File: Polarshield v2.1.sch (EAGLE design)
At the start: 82 parts, among them CN1 1X4-CLEANBIG, CN2 1X4-CLEANBIG, CN3 1X4-CLEANBIG, CN4 1X4-CLEANBIG, CN5 1X4-CLEANBIG, CN6 1X4-CLEANBIG, IC1 MP2307, IC2 74541PW, IC3 74541PW, IC4 74541PW, IC5 74541PW, J1 1X2-3.5MM, U1 ARDUINO_MEGA_SHIELD, X1 2.1MMJACKTHM

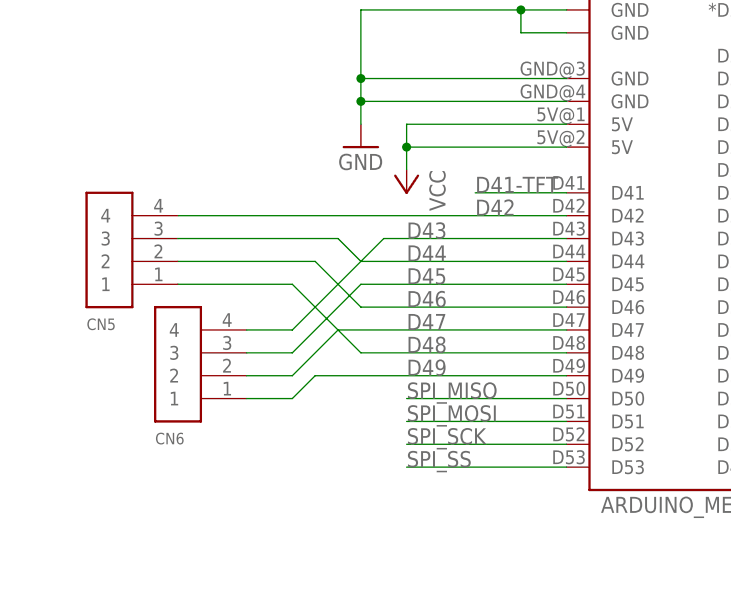
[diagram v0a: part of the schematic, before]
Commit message: Ran the DRU, ready for making.
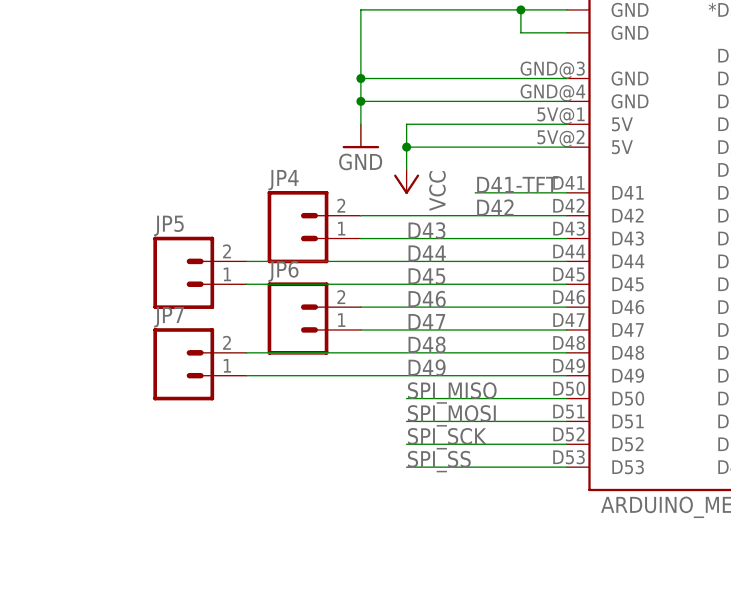
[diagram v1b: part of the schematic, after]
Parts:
- removed CN5, CN6: 1X4-CLEANBIG, Polarshield v2.0e:1X4-CLEANBIG
- added JP4, JP5, JP6, JP7: (no value), SparkFun-Connectors:M02POGO_PIN_HOLES_ONLY
- JP1, JP3: device SparkFun-Connectors:M021X02_NO_SILK -> SparkFun-Connectors:M02POGO_PIN_HOLES_ONLY
- JP2: device SparkFun-Connectors:M031X03_NO_SILK -> SparkFun-Connectors:M03POGO_PIN_HOLES_ONLY
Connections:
- net D42: now also JP4.2; no longer CN5.4
- net D43: now also JP4.1; no longer CN6.4
- net D44: now also JP5.2; no longer CN5.3
- net D45: now also JP5.1; no longer CN6.3
- net D46: now also JP6.2; no longer CN5.2
- net D47: now also JP6.1; no longer CN6.2
- net D48: now also JP7.2; no longer CN5.1
- net D49: now also JP7.1; no longer CN6.1
